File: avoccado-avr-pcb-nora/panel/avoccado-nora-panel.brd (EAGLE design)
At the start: 50 x 50 mm, 51 parts, among them Q1 16MHz, Q2 FET, U2 MCP73831

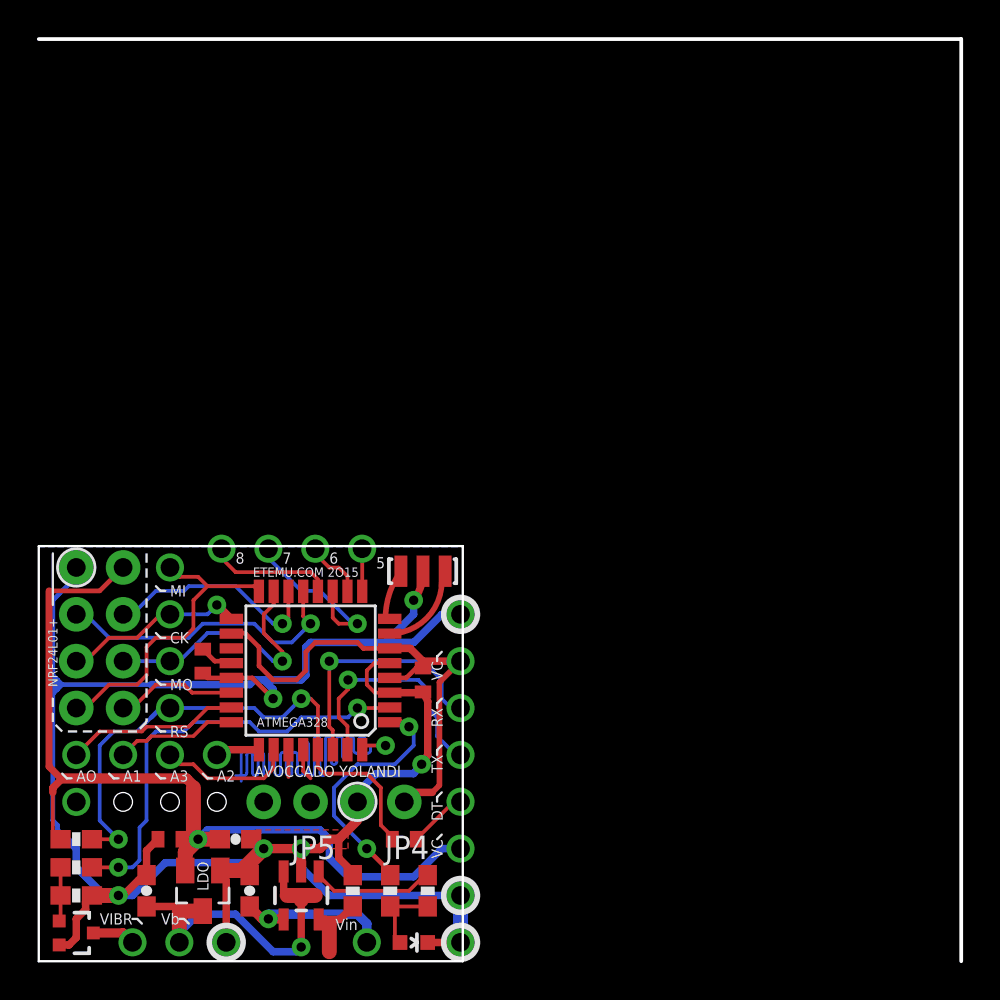
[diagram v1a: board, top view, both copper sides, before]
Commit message: add rectangles at plated half holes
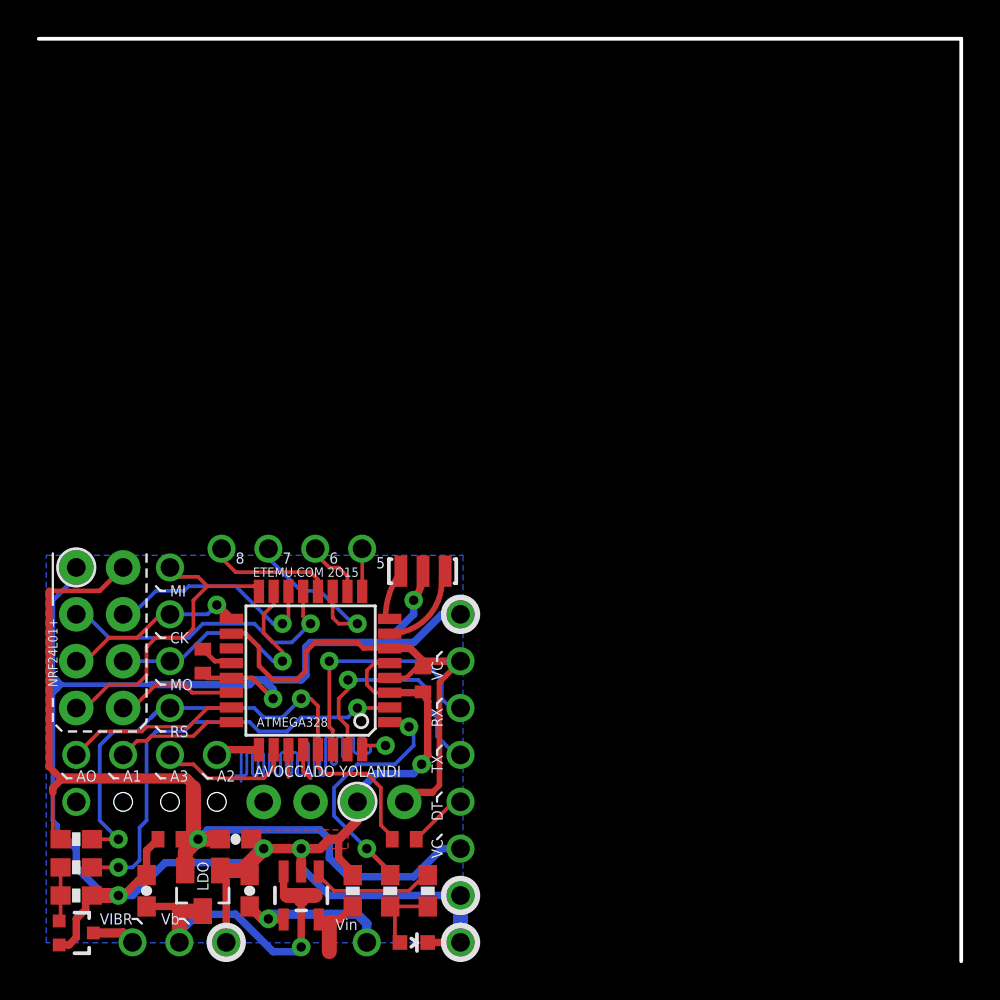
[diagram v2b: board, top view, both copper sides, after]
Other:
- outline, holes or cut-outs redrawn
- board text added: "3.3V 3.6-4.2V 5-5.5V"
- board text added: "SHURE OPEN TECHNOLOGIES AVOCCADO AVR NORA 1 ETEMU.COM 2015"
- board text added: "Vc Vb Vi"
- board text added: "Vin max 5V"
- board text removed: "SHURE OPEN TECHNOLOGIES AVOCCADO AVR YOLANDI V1 ETEMU.COM 2014"
- board text removed: "Vin 5V"
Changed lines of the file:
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@@
 <setting verticaltext="up"/>
 </settings>
-<grid distance="0.02" unitdist="inch" unit="inch" style="lines" multiple="1" display="yes" altdistance="0.01" altunitdist="inch" altunit="inch"/>
+<grid distance="1" unitdist="mm" unit="mm" style="lines" multiple="1" display="yes" altdistance="0.1" altunitdist="mm" altunit="mm"/>
 <layers>
-<layer number="1" name="Top" color="5" fill="1" visible="yes" active="yes"/>
+<layer number="1" name="Top" color="5" fill="1" visible="no" active="yes"/>
 <layer number="2" name="Route2" color="1" fill="3" visible="no" active="no"/>
 <layer number="3" name="Route3" color="4" fill="3" visible="no" active="no"/>
@@
 <layer number="19" name="Unrouted" color="6" fill="1" visible="yes" active="yes"/>
 <layer number="20" name="Dimension" color="15" fill="1" visible="yes" active="yes"/>
-<layer number="21" name="tPlace" color="16" fill="1" visible="yes" active="yes"/>
+<layer number="21" name="tPlace" color="16" fill="1" visible="no" active="yes"/>
 <layer number="22" name="bPlace" color="6" fill="1" visible="yes" active="yes"/>
-<layer number="23" name="tOrigins" color="15" fill="1" visible="yes" active="yes"/>
+<layer number="23" name="tOrigins" color="15" fill="1" visible="no" active="yes"/>
 <layer number="24" name="bOrigins" color="15" fill="1" visible="yes" active="yes"/>
 <layer number="25" name="tNames" color="7" fill="1" visible="no" active="yes"/>
-<layer number="26" name="bNames" color="7" fill="1" visible="no" active="yes"/>
+<layer number="26" name="bNames" color="7" fill="1" visible="yes" active="yes"/>
 <layer number="27" name="tValues" color="7" fill="1" visible="no" active="yes"/>
-<layer number="28" name="bValues" color="7" fill="1" visible="no" active="yes"/>
+<layer number="28" name="bValues" color="7" fill="1" visible="yes" active="yes"/>
 <layer number="29" name="tStop" color="7" fill="3" visible="no" active="yes"/>
 <layer number="30" name="bStop" color="7" fill="6" visible="no" active="yes"/>
@@
 <layer number="43" name="vRestrict" color="2" fill="10" visible="no" active="yes"/>
 <layer number="44" name="Drills" color="7" fill="1" visible="no" active="yes"/>
-<layer number="45" name="Holes" color="7" fill="1" visible="yes" active="yes"/>
+<layer number="45" name="Holes" color="7" fill="1" visible="no" active="yes"/>
 <layer number="46" name="Milling" color="3" fill="1" visible="no" active="yes"/>
 <layer number="47" name="Measures" color="7" fill="1" visible="no" active="yes"/>
@@
 <layer number="49" name="Reference" color="7" fill="1" visible="no" active="yes"/>
 <layer number="50" name="dxf" color="7" fill="1" visible="no" active="yes"/>
-<layer number="51" name="tDocu" color="6" fill="1" visible="yes" active="yes"/>
-<layer number="52" name="bDocu" color="7" fill="1" visible="no" active="yes"/>
+<layer number="51" name="tDocu" color="6" fill="1" visible="no" active="yes"/>
+<layer number="52" name="bDocu" color="7" fill="1" visible="yes" active="yes"/>
 <layer number="53" name="tGND_GNDA" color="7" fill="9" visible="no" active="no"/>
 <layer number="54" name="bGND_GNDA" color="1" fill="9" visible="no" active="no"/>
@@
 Yolandi is the minified version of Avoccado-avr with less pins broken out and a footprint of less than one square inch for the PCB without peripherals.</description>
 <plain>
-<wire x1="50" y1="0" x2="50" y2="49.984" width="0.2032" layer="20"/>
-<wire x1="50" y1="49.984" x2="0" y2="49.984" width="0.2032" layer="20"/>
+<wire x1="50" y1="0" x2="50" y2="50" width="0.2032" layer="20"/>
+<wire x1="50" y1="50" x2="0" y2="50" width="0.2032" layer="20"/>
 <text x="11.811" y="12.708" size="0.508" layer="21" font="vector">ATMEGA328</text>
 <circle x="17.78" y="6.104" radius="0.254" width="0.508" layer="30"/>
@@
 <wire x1="0.762" y1="12.962" x2="0.762" y2="14.486" width="0.127" layer="21" style="shortdash"/>
 <wire x1="0.762" y1="19.312" x2="0.762" y2="22.106" width="0.127" layer="21"/>
-<wire x1="0" y1="0" x2="22.984" y2="0" width="0.127" layer="20"/>
-<wire x1="22.984" y1="0" x2="22.984" y2="22.5" width="0.127" layer="20"/>
-<wire x1="22.984" y1="22.5" x2="0" y2="22.5" width="0.127" layer="20"/>
-<wire x1="0" y1="22.5" x2="0" y2="0" width="0.127" layer="20"/>
-<text x="22.568" y="21.725" size="0.6096" layer="22" font="vector" rot="MR0" align="top-left">WARNING
-DO NOT SWALLOW THIS PRODUCT</text>
-<text x="21.336" y="5.215" size="0.6096" layer="22" font="vector" rot="MR0" align="top-left">SHURE OPEN TECHNOLOGIES
-AVOCCADO AVR YOLANDI V1
-ETEMU.COM 2014</text>
+<text x="20.568" y="20.725" size="0.6096" layer="22" font="vector" rot="MR0" align="top-left">WARNING
+DO NOT SWALLOW
+THIS PRODUCT</text>
+<text x="20.636" y="7.015" size="0.8128" layer="22" font="vector" ratio="10" rot="MR0" align="top-left">SHURE OPEN TECHNOLOGIES
+AVOCCADO AVR NORA 1
+ETEMU.COM 2015</text>
 <text x="0.762" y="20.709" size="0.508" layer="22" font="vector" rot="MR270" align="center-left">NRF24L01+</text>
 <wire x1="5.842" y1="22.106" x2="5.842" y2="12.962" width="0.127" layer="22" style="longdash"/>
@@
 <text x="7.443759375" y="3.314603125" size="1.778" layer="22" font="vector" ratio="15" rot="MR0" align="center">+</text>
 <text x="9.993371875" y="3.320159375" size="1.778" layer="22" font="vector" ratio="15" rot="MR0" align="center">-</text>
-<text x="4.064" y="2.294" size="0.6096" layer="22" ratio="10" rot="SMR0" align="center-right">VIBR</text>
-<text x="14.02029375" y="1.97400625" size="0.6096" layer="22" ratio="10" rot="SMR0" align="center-right">Vin 5V</text>
+<text x="4.064" y="2.494" size="0.6096" layer="22" ratio="10" rot="SMR0" align="center-right">VIBR</text>
+<text x="15.02029375" y="2.47400625" size="0.6096" layer="22" ratio="10" rot="SMR0" align="center-right">Vin max 5V</text>
 <text x="21.59" y="13.724" size="0.6096" layer="22" ratio="10" rot="MR90" align="center-right">RX</text>
 <wire x1="21.59" y1="13.724" x2="21.59" y2="13.978" width="0.127" layer="22"/>
@@
 <text x="15.748" y="21.836" size="0.6096" layer="22" ratio="10" rot="SMR180" align="center-left">6</text>
 <text x="18.288" y="21.836" size="0.6096" layer="22" ratio="10" rot="SMR180" align="center-left">5</text>
-<text x="7.694484375" y="2.497475" size="0.6096" layer="22" ratio="10" rot="SMR0" align="center-right">LiPo</text>
+<text x="7.794484375" y="2.497475" size="0.6096" layer="22" ratio="10" rot="SMR0" align="center-right">LiPo</text>
 <hole x="4.572" y="8.636" drill="1.016"/>
 <hole x="7.112" y="8.636" drill="1.016"/>
 <hole x="9.652" y="8.636" drill="1.016"/>
+<text x="19.168" y="15.025" size="0.6096" layer="22" font="vector" rot="MR0">3.3V
+3.6-4.2V
+5-5.5V</text>
+<text x="20.568" y="15.025" size="0.6096" layer="22" font="vector" rot="MR0">Vc
+Vb
+Vi</text>
+<wire x1="16.896" y1="1.49" x2="15.742" y2="1.49" width="0.127" layer="22"/>
+<wire x1="15.742" y1="1.49" x2="15.488" y2="1.744" width="0.127" layer="22"/>
+<wire x1="19.62" y1="1.454" x2="19.874" y2="1.708" width="0.127" layer="22"/>
+<wire x1="18.666" y1="1.454" x2="19.62" y2="1.454" width="0.127" layer="22"/>
+<text x="4.993371875" y="3.320159375" size="1.016" layer="22" font="vector" ratio="15" rot="MR0" align="center">-</text>
 </plain>
 <attributes>
@@
 <element name="JP28" library="SparkFun-Connectors" package="1X02_NO_SILK" value="M021X02_NO_SILK" x="2.032" y="16.264" smashed="yes"/>
 <element name="JP29" library="SparkFun-Connectors" package="1X02_NO_SILK" value="M021X02_NO_SILK" x="2.032" y="13.724" smashed="yes"/>
-<element name="JP4" library="SparkFun-Connectors" package="1X02_NO_SILK" value="M021X02_NO_SILK" x="19.812" y="8.636" rot="R180"/>
-<element name="JP5" library="SparkFun-Connectors" package="1X02_NO_SILK" value="M021X02_NO_SILK" x="14.732" y="8.636" rot="R180"/>
-<element name="TP2" library="SparkFun-Connectors" package="1X01NS-KIT" value="M01NOSILK-KIT" x="2.032" y="8.636"/>
+<element name="JP4" library="SparkFun-Connectors" package="1X02_NO_SILK" value="M021X02_NO_SILK" x="19.812" y="8.636" smashed="yes" rot="R180"/>
+<element name="JP5" library="SparkFun-Connectors" package="1X02_NO_SILK" value="M021X02_NO_SILK" x="14.732" y="8.636" smashed="yes" rot="R180"/>
+<element name="TP2" library="SparkFun-Connectors" package="1X01NS-KIT" value="M01NOSILK-KIT" x="2.032" y="8.636" smashed="yes"/>
 </elements>
 <signals>
@@
 <contactref element="AVR" pad="3"/>
 <contactref element="AVR" pad="5"/>
-<polygon width="0.2032" layer="16" isolate="0.3048">
-<vertex x="0" y="22.458"/>
-<vertex x="22.972" y="22.458"/>
-<vertex x="22.972" y="0"/>
-<vertex x="0" y="0"/>
+<polygon width="0.2032" layer="16" isolate="0.2794">
+<vertex x="0.4" y="22"/>
+<vertex x="23" y="22"/>
+<vertex x="23" y="1"/>
+<vertex x="0.4" y="1"/>
 </polygon>
 <contactref element="LDO" pad="1"/>
